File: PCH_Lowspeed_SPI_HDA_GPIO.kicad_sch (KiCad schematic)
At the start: 1 part

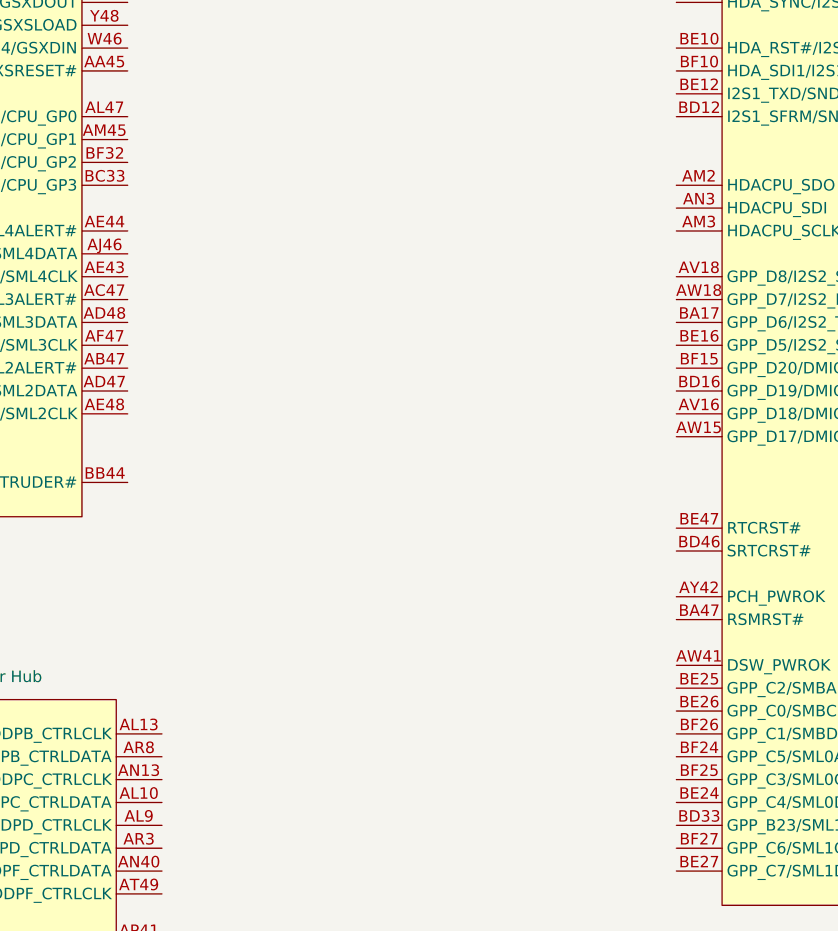
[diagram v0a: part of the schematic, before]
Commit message: Some DP and power work
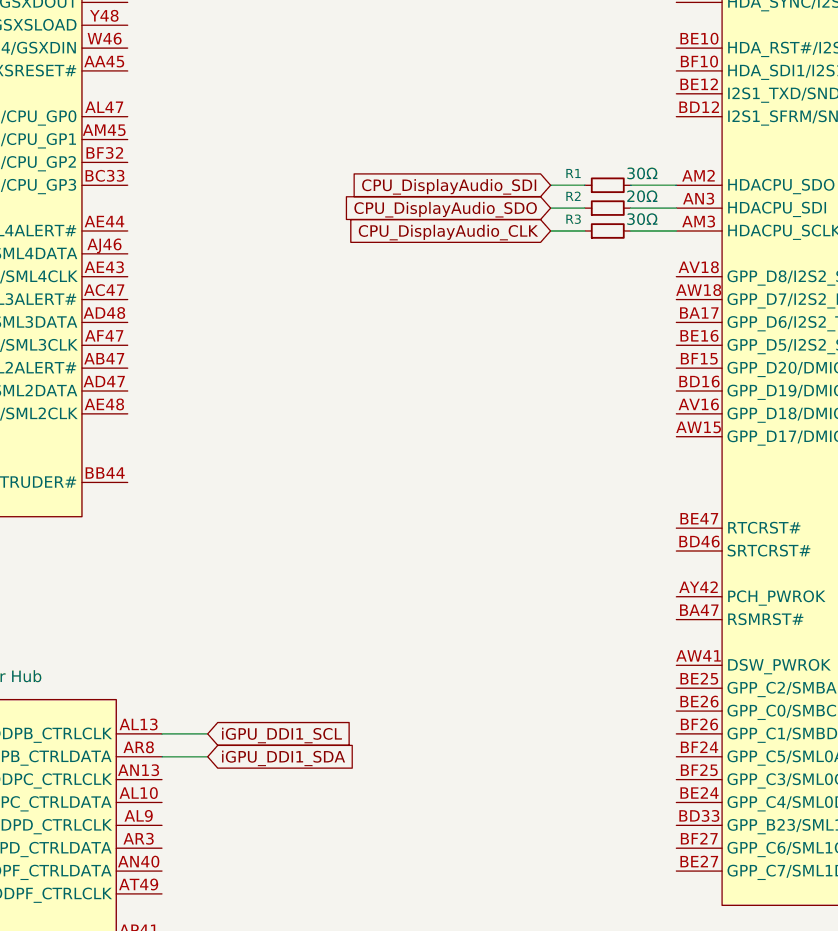
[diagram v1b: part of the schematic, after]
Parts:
- added R1, R3: 30Ω, Resistor_SMD:R_0402_1005Metric, symbol Device:R_Small
- added R2: 20Ω, Resistor_SMD:R_0402_1005Metric, symbol Device:R_Small
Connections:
- net iGPU_DDI1_SCL: now reaches UPCH1.AL13 (GPP_I5/DDPB_CTRLCLK)
- net iGPU_DDI1_SDA: now reaches UPCH1.AR8 (GPP_I6/DDPB_CTRLDATA)
- net at UPCH1.AM2 (HDACPU_SDO): now also R1.2
- net at UPCH1.AM3 (HDACPU_SCLK): now also R3.2
- net at UPCH1.AN3 (HDACPU_SDI): now also R2.2
- new net CPU_DisplayAudio_CLK: R3.1
- new net CPU_DisplayAudio_SDI: R1.1
- new net CPU_DisplayAudio_SDO: R2.1

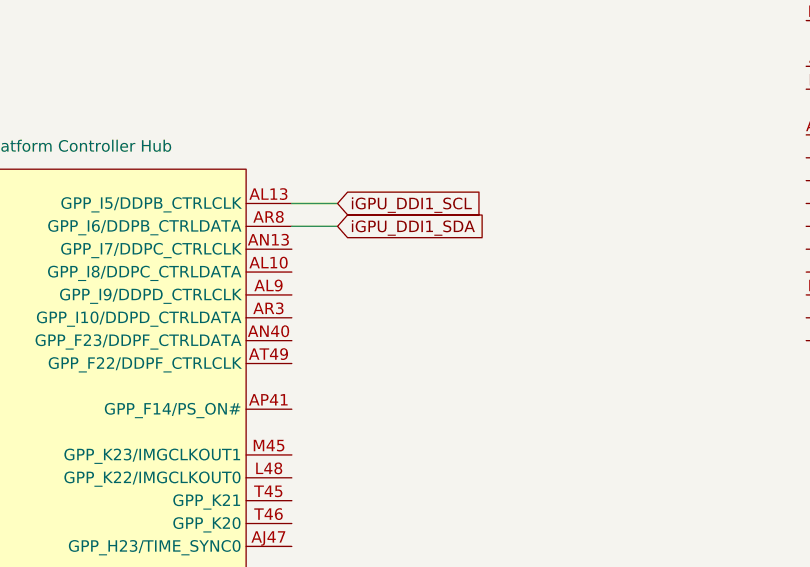
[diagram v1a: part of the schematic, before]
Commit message: More DP
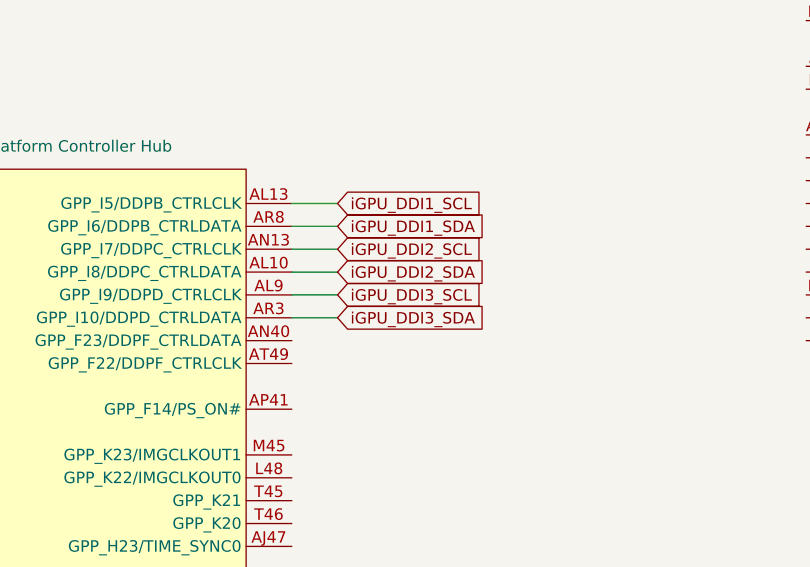
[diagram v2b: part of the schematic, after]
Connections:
- net iGPU_DDI2_SDA: now reaches UPCH1.AL10 (GPP_I8/DDPC_CTRLDATA)
- net iGPU_DDI3_SCL: now reaches UPCH1.AL9 (GPP_I9/DDPD_CTRLCLK)
- net iGPU_DDI2_SCL: now reaches UPCH1.AN13 (GPP_I7/DDPC_CTRLCLK)
- net iGPU_DDI3_SDA: now reaches UPCH1.AR3 (GPP_I10/DDPD_CTRLDATA)
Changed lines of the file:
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@@
+	(wire
+		(pts
+			(xy 120.65 123.19) (xy 115.57 123.19)
+		)
+		(stroke
+			(width 0)
+			(type default)
+		)
+	)
 	(wire
 		(pts
@@
 	(wire
 		(pts
+			(xy 120.65 130.81) (xy 115.57 130.81)
+		)
+		(stroke
+			(width 0)
+			(type default)
+		)
+	)
+	(wire
+		(pts
+			(xy 120.65 128.27) (xy 115.57 128.27)
+		)
+		(stroke
+			(width 0)
+			(type default)
+		)
+	)
+	(wire
+		(pts
+			(xy 120.65 125.73) (xy 115.57 125.73)
+		)
+		(stroke
+			(width 0)
+			(type default)
+		)
+	)
+	(wire
+		(pts
 			(xy 158.75 57.15) (xy 162.56 57.15)
 		)
@@
 		)
 	)
+	(global_label "iGPU_DDI3_SDA"
+		(shape input)
+		(at 120.65 130.81 0)
+		(fields_autoplaced yes)
+		(effects
+			(font
+				(size 1.27 1.27)
+			)
+			(justify left)
+		)
+		(property "Intersheetrefs" "${INTERSHEET_REFS}"
+			(at 144.9831 130.81 0)
+			(effects
+				(font
+					(size 1.27 1.27)
+				)
+				(justify left)
+				(hide yes)
+			)
+		)
+	)
+	(global_label "iGPU_DDI2_SCL"
+		(shape input)
+		(at 120.65 123.19 0)
+		(fields_autoplaced yes)
+		(effects
+			(font
+				(size 1.27 1.27)
+			)
+			(justify left)
+		)
+		(property "Intersheetrefs" "${INTERSHEET_REFS}"
+			(at 144.9831 123.19 0)
+			(effects
+				(font
+					(size 1.27 1.27)
+				)
+				(justify left)
+				(hide yes)
+			)
+		)
+	)
 	(global_label "CPU_DisplayAudio_CLK"
 		(shape input)
@@
 		)
 	)
+	(global_label "iGPU_DDI3_SCL"
+		(shape input)
+		(at 120.65 128.27 0)
+		(fields_autoplaced yes)
+		(effects
+			(font
+				(size 1.27 1.27)
+			)
+			(justify left)
+		)
+		(property "Intersheetrefs" "${INTERSHEET_REFS}"
+			(at 144.9831 128.27 0)
+			(effects
+				(font
+					(size 1.27 1.27)
+				)
+				(justify left)
+				(hide yes)
+			)
+		)
+	)
 	(global_label "iGPU_DDI1_SCL"
 		(shape input)
@@
 			(effects
 				(font
+					(size 1.27 1.27)
+				)
+				(justify left)
+				(hide yes)
+			)
+		)
+	)
+	(global_label "iGPU_DDI2_SDA"
+		(shape input)
+		(at 120.65 125.73 0)
+		(fields_autoplaced yes)
+		(effects
+			(font
+				(size 1.27 1.27)
+			)
+			(justify left)
+		)
+		(property "Intersheetrefs" "${INTERSHEET_REFS}"
+			(at 144.9831 125.73 0)
+			(effects
+				(font
